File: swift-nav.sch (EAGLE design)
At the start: 110 parts, among them J1 SMA, J3 SMA, J4 PIN_HDR_EDG_1.27MM_5-2, J6 ZX62-B-5PA, U1 6SLX9FTG256, U10 MAX2769, U12 PT7M8206B33TA5EX, U13 M25PX80, U2 LTC3407A, U3 STM32-M-64-LQFP, U4 7Q-16.368MBG-T, U8 B4050, X3 FPGA_DEBUG_HDR

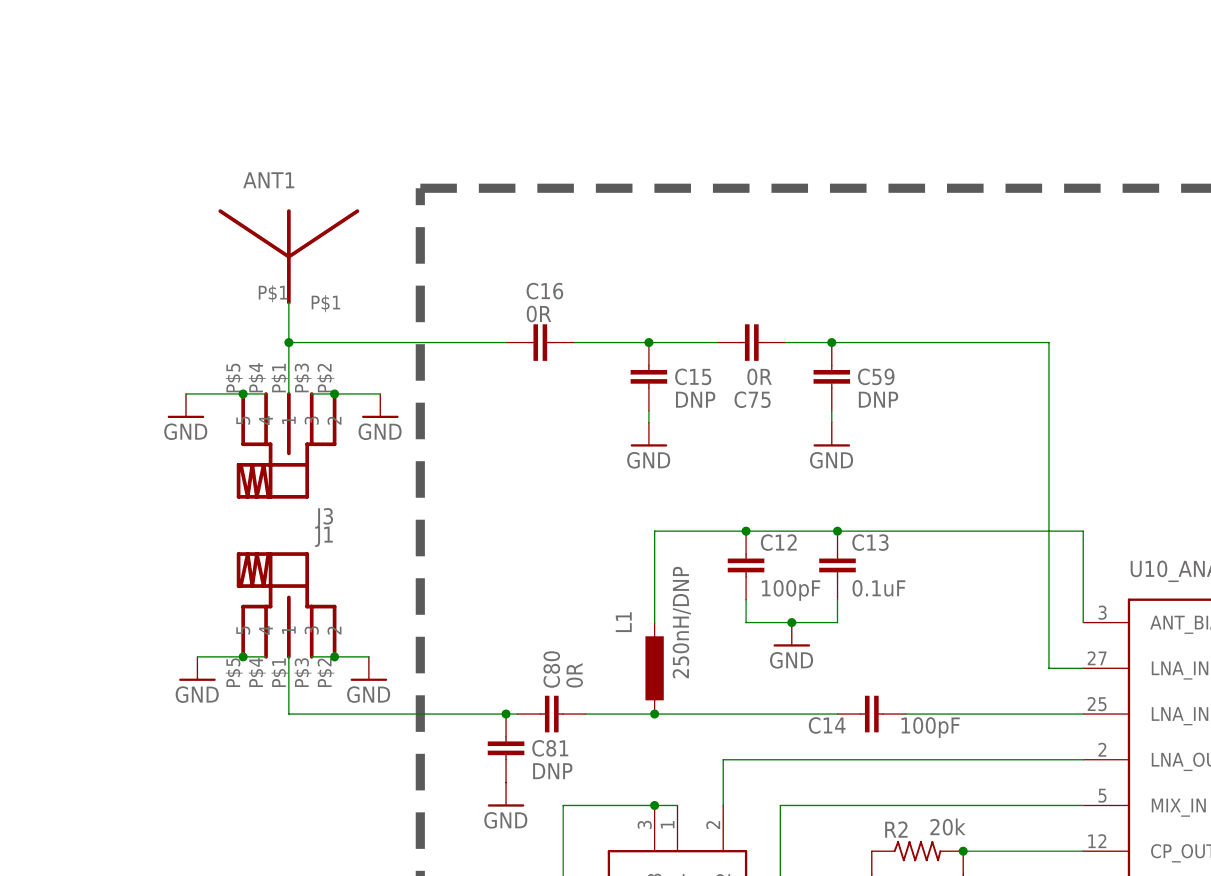
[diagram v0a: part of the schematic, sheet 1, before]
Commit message: Working on the layout
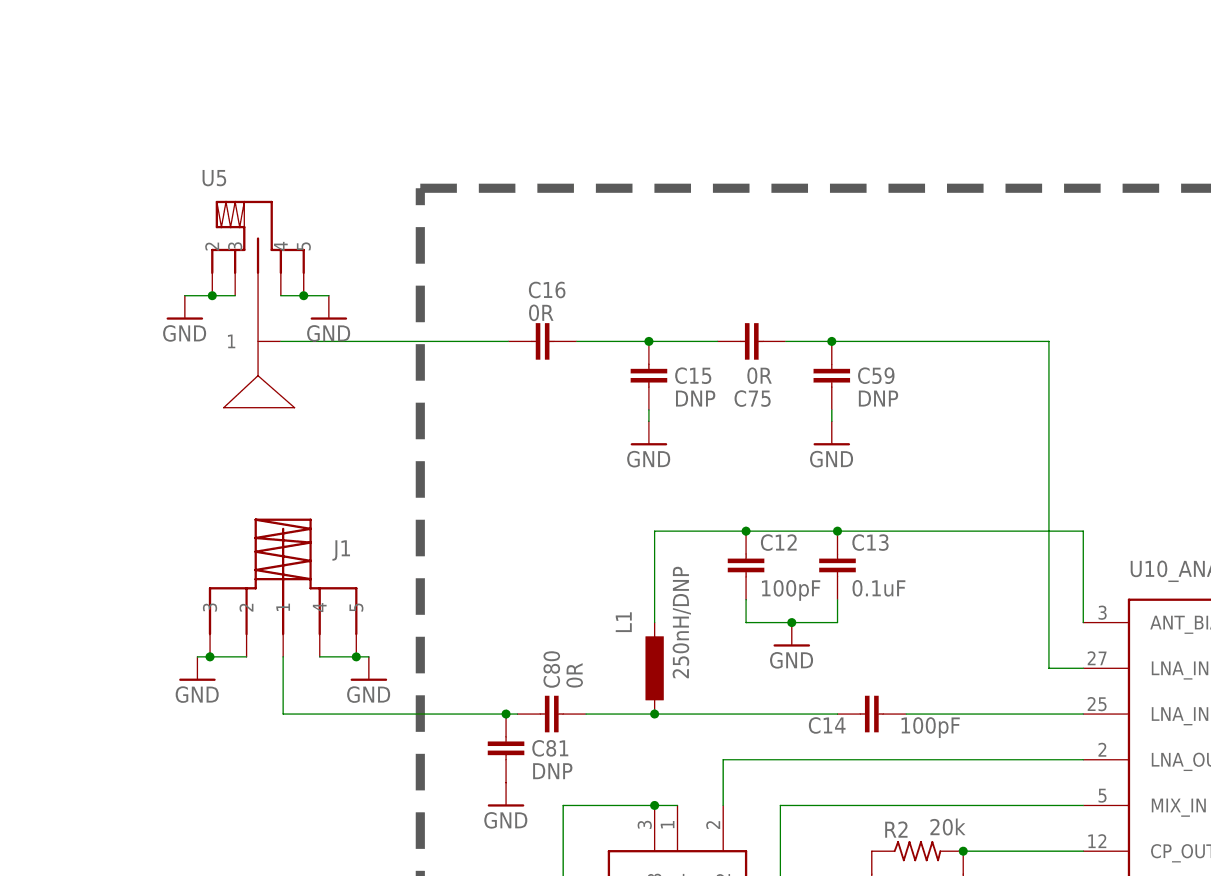
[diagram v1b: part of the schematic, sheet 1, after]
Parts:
- removed ANT1: GPS_PATCH_ANTENNA, joby_robotics:GPS_PATCH_ANTENNA
- removed J3: SMA, joby_robotics:SMA
- added U5: SMA_PATCH, joby_robotics:SMA_PATCH
- J1: value SMA -> SMA_EDGE; device joby_robotics:SMA -> swift-nav:SMA_EDGE
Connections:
- removed net N$45: ANT1.P$1, C16.2, J3.1
- new net 3: J1.2, J1.3
- new net 4: U5.4, U5.5
- new net 5: J1.4, J1.5
- new net N$14: C16.2, U5.1
- net GND: now also U5.2, U5.3; no longer J1.2, J1.3, J1.4, J1.5, J3.2, J3.3, J3.4, J3.5
